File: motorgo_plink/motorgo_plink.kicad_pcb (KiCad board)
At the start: 4 copper layers, 80.2 x 56 mm, 142 parts, among them J1 USB4520-03-0-A_REVA, J10 Conn_01x02_Pin, J12 USB4520-03-0-A_REVA, J13 I2C_STANDARDQWIIC, J14 BM05B-SRSS-TB_LF__SN_, J15 I2C_STANDARDQWIIC, J16 BM05B-SRSS-TB_LF__SN_, J17 I2C_STANDARDQWIIC, J18 BM05B-SRSS-TB_LF__SN_, J19 I2C_STANDARDQWIIC, J20 BM05B-SRSS-TB_LF__SN_, J22 Conn_01x02_Pin, J23 Conn_01x06_Pin, J4 Conn_02x20_Odd_Even, J5 Conn_02x20_Odd_Even, J6 Conn_01x02_Pin, J8 Conn_01x02_Pin, Q1 SI2323, U1 ESP32-S3-WROOM-1, U10 LIS3MDLTR, U11 LSM6DS3TR, U2 USBLC6-2P6, U3 DRV8874PWPR, U4 DRV8874PWPR, U5 DRV8874PWPR, U6 TPS54620RHLR, U7 HUSB238_002DD, U8 AMS1117-3.3, U9 DRV8874PWPR

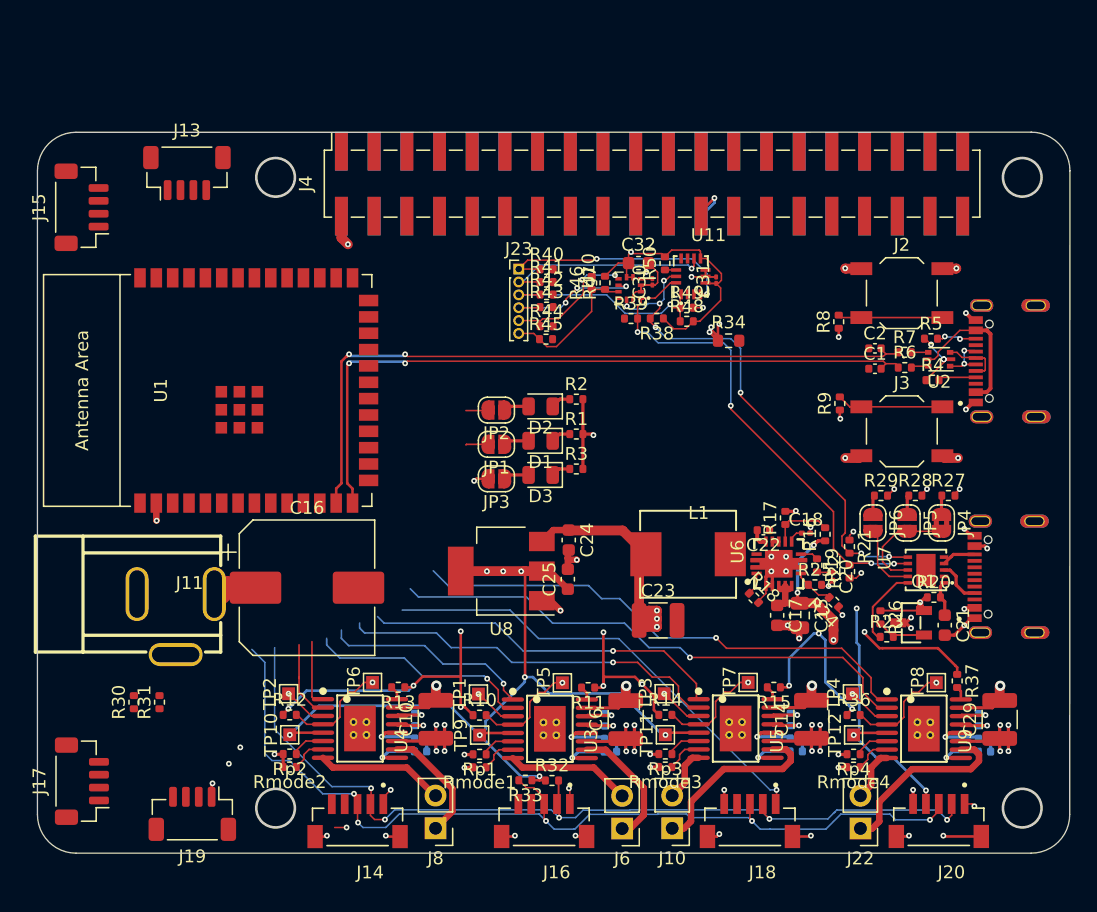
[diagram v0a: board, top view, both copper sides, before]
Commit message: WIP update. change USBC port
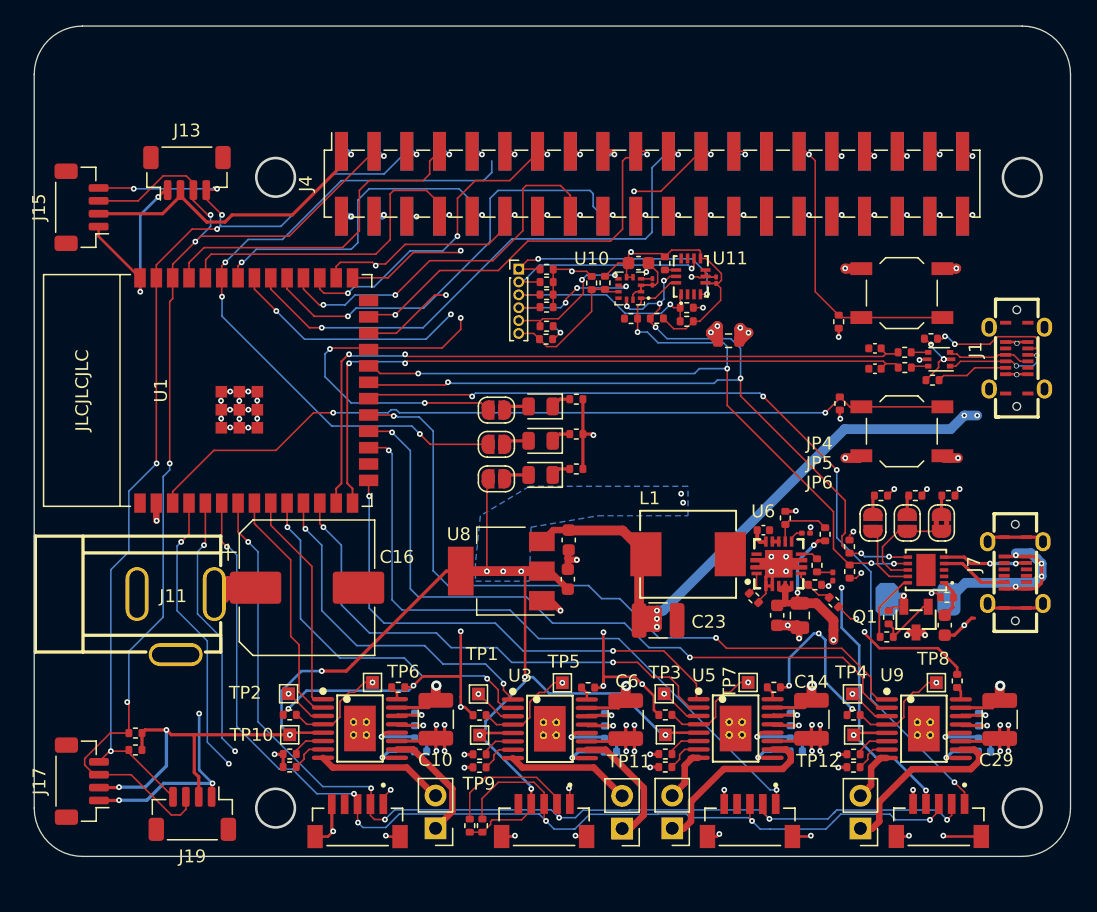
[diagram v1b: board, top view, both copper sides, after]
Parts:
- removed J12: USB4520-03-0-A_REVA, mg_mini_v1r3:GCT_USB4520-03-0-A_REVA
- added D4: 20V 5A, LCSC_parts:D_SMB_LCSC_C5366311, B.Cu at (162.9, 96.3)
- added J7: USB4520-03-0-A_REVA, mg_mini_v1r3:USB-C-SMD_TYPEC-303-ACP16, F.Cu at (170.5, 94.2)
- J1: footprint mg_mini_v1r3:GCT_USB4520-03-0-A_REVA -> mg_mini_v1r3:USB-C-SMD_TYPEC-303-ACP16
- Rp1, Rp2, Rp3, Rp4: value 4.83k -> 4.87k
- moved R32 7.29 mm to (128.1, 113.9), turned to 90 degrees
- moved R33 4.86 mm to (129.1, 113.9), turned to 90 degrees
- moved R31 4.16 mm to (102.1, 108.0), turned to 180 degrees
- moved R30 2.40 mm to (102.1, 106.7), turned to 180 degrees
- moved J1 1.98 mm to (170.6, 77.5)
- moved R20 1.02 mm to (165.2, 96.1)
- moved R26 0.64 mm to (160.6, 97.7)
- moved Q1 0.45 mm to (162.7, 97.9), turned to 90 degrees
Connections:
- J4 pad 10: gpio43 -> gpio44
- J4 pad 8: gpio44 -> gpio43
- J5 pad 7: gpio44 -> gpio43
- J5 pad 9: gpio43 -> gpio44
- Q1 pad 2: +VDC -> Net-(D4-K)
- R26 pad 1: +VDC -> Net-(D4-K)
- U1 pad 10: m3_PH -> m2_PH
- U1 pad 11: m4_EN -> m2_EN
- U1 pad 12: gpio8 -> m3_PH
- U1 pad 15: gpio3 -> m3_EN
- U1 pad 17: gpio9 -> m3_enc_cs
- U1 pad 18: m1_EN -> m4_PH
- U1 pad 19: m1_PH -> m4_EN
- U1 pad 20: m2_EN -> m4_enc_cs
- U1 pad 21: m2_PH -> hidden_sda
- U1 pad 22: m3_EN -> hidden_scl
- U1 pad 23: m4_PH -> gpio38
- U1 pad 24: gpio47 -> gpio41
- U1 pad 25: m2_enc_cs -> gpio42
- U1 pad 28: enc_sda -> gpio4
- U1 pad 29: enc_scl -> gpio7
- U1 pad 30: m1_enc_cs -> gpio3
- U1 pad 31: gpio38 -> gpio8
- U1 pad 34: gpio41 -> gpio44
- U1 pad 35: gpio42 -> gpio47
- U1 pad 36: gpio44 -> gpio43
- U1 pad 37: gpio43 -> gpio9
- U1 pad 4: gpio4 -> m2_enc_cs
- U1 pad 5: hidden_scl -> m1_enc_cs
- U1 pad 6: hidden_sda -> enc_sda
- U1 pad 7: gpio7 -> enc_scl
- U1 pad 8: m3_enc_cs -> m1_PH
- U1 pad 9: m4_enc_cs -> m1_EN
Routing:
- net +3.3V: track 117.9 -> 211.8 mm, vias 18 -> 24
- net sda: track 0.00 -> 88.5 mm, vias 0 -> 5
- net scl: track 0.00 -> 85.5 mm, vias 0 -> 7
- net GND: track 93.0 -> 165.8 mm, vias 52 -> 75
- net boot: track 8.13 -> 64.4 mm, vias 0 -> 2
- net reset: track 8.29 -> 64.3 mm, vias 0 -> 2
- net gpio47: track 1.74 -> 55.3 mm, vias 0 -> 4
- net gpio38: track 5.40 -> 53.1 mm, vias 1 -> 4
- net gpio40: track 0.00 -> 47.1 mm, vias 0 -> 4
- net gpio39: track 0.00 -> 43.3 mm, vias 0 -> 2
- net gpio8: track 0.00 -> 35.3 mm, vias 0 -> 2
- net gpio41: track 0.00 -> 33.9 mm, vias 0 -> 2
- net gpio3: track 0.00 -> 31.4 mm, vias 0 -> 3
- net gpio42: track 0.00 -> 31.2 mm, vias 0 -> 2
- net hidden_sda: track 40.4 -> 69.6 mm, vias 7 -> 8
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- added copper zone on B.Cu, net +3.3V
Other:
- board size 80.2 x 56 mm -> 80.5 x 64.5 mm
